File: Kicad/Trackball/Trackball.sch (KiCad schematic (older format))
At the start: 23 parts, among them J1 52559-1233, J10 Conn_01x04_Female, J11 Conn_01x04_Female, J12 Conn_01x04_Female, J13 Conn_01x04_Female, J14 Conn_01x04_Female, J15 Conn_01x04_Female, J16 Conn_01x04_Female, J17 Conn_01x04_Female, J2 Conn_01x04_Male, J3 Conn_01x04_Male, J4 Conn_01x04_Male, J5 Conn_01x04_Male, J6 Conn_01x04_Male, J7 Conn_01x04_Male, J8 Conn_01x04_Male, J9 Conn_01x04_Male, U1 ProMicro

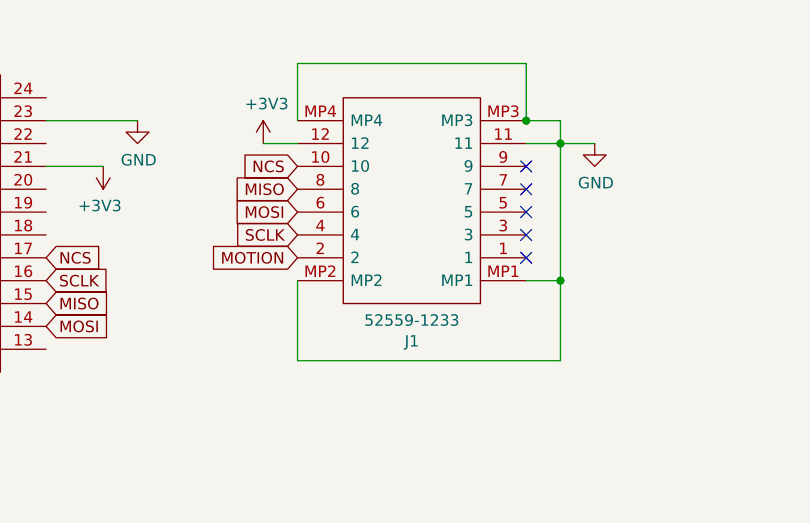
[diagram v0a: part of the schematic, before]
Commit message: Trackball v2: Initial project draft, lot of changes coming.
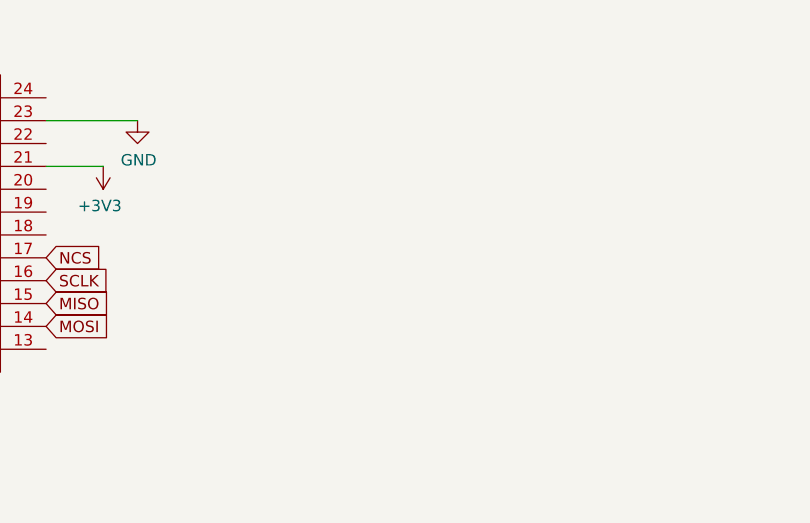
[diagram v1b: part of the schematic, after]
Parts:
- removed J1: 52559-1233, 52559-1233:525591233, symbol 52559-1233:52559-1233
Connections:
- no-connect marks 5 -> 0
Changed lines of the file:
@@
 $EndComp
-$Comp
-L power:+3V3 #PWR0101
-U 1 1 681FE87E
-P 6850 2800
-F 0 "#PWR0101" H 6850 2650 50  0001 C CNN
-F 1 "+3V3" H 6865 2973 50  0000 C CNN
-F 2 "" H 6850 2800 50  0001 C CNN
-F 3 "" H 6850 2800 50  0001 C CNN
-	1    6850 2800
-	1    0    0    -1
-$EndComp
-Wire Wire Line
-	7000 2800 6850 2800
-$Comp
-L power:GND #PWR0102
-U 1 1 68201B1F
-P 8300 2800
-F 0 "#PWR0102" H 8300 2550 50  0001 C CNN
-F 1 "GND" H 8305 2627 50  0000 C CNN
-F 2 "" H 8300 2800 50  0001 C CNN
-F 3 "" H 8300 2800 50  0001 C CNN
-	1    8300 2800
-	1    0    0    -1
-$EndComp
-Text GLabel 7000 2900 0    50   Input ~ 0
-NCS
-Text GLabel 7000 3000 0    50   Input ~ 0
-MISO
-Text GLabel 7000 3100 0    50   Input ~ 0
-MOSI
-Text GLabel 7000 3200 0    50   Input ~ 0
-SCLK
-Text GLabel 7000 3300 0    50   Input ~ 0
-MOTION
-Wire Wire Line
-	8000 3400 8150 3400
-Wire Wire Line
-	8150 2700 8000 2700
-Wire Wire Line
-	8000 2700 8000 2450
-Wire Wire Line
-	8000 2450 7000 2450
-Wire Wire Line
-	7000 2450 7000 2700
-Wire Wire Line
-	7000 3750 8150 3750
-Wire Wire Line
-	8150 3750 8150 3400
 $Comp
 L MX_Alps_Hybrid:MX-NoLED MX4
@@
 	-1   0    0    -1
 $EndComp
-Wire Wire Line
-	8000 2800 8150 2800
-Connection ~ 8150 3400
-Wire Wire Line
-	8150 2700 8150 2800
-Connection ~ 8150 2800
-Wire Wire Line
-	8150 2800 8300 2800
-Wire Wire Line
-	8150 2800 8150 3400
 Text GLabel 4500 2700 0    50   Input ~ 0
 MOTION
@@
 Wire Wire Line
 	5900 2900 6150 2900
-Connection ~ 8000 2700
-Wire Wire Line
-	7000 3400 7000 3750
-$Comp
-L 52559-1233:52559-1233 J1
-U 1 1 681FC9A0
-P 8000 3400
-F 0 "J1" H 8500 3665 50  0000 C CNN
-F 1 "52559-1233" H 8500 3574 50  0000 C CNN
-F 2 "52559-1233:525591233" H 8850 3500 50  0001 L CNN
-F 3 "" H 8850 3400 50  0001 L CNN
-F 4 "FFC & FPC Connectors 0.5 FPC ZIF 12Ckt Sn-Ag-Bi" H 8850 3300 50  0001 L CNN "Description"
-F 5 "5.55" H 8850 3200 50  0001 L CNN "Height"
-F 6 "538-52559-1233" H 8850 3100 50  0001 L CNN "Mouser Part Number"
-F 7 "https://www.mouser.co.uk/ProductDetail/Molex/52559-1233?qs=Q7nJoqLg%252BZgmtCe8OD7vZw%3D%3D" H 8850 3000 50  0001 L CNN "Mouser Price/Stock"
-F 8 "Molex" H 8850 2900 50  0001 L CNN "Manufacturer_Name"
-F 9 "52559-1233" H 8850 2800 50  0001 L CNN "Manufacturer_Part_Number"
-	1    8000 3400
-	-1   0    0    1
-$EndComp
-NoConn ~ 8000 2900
-NoConn ~ 8000 3000
-NoConn ~ 8000 3100
-NoConn ~ 8000 3200
-NoConn ~ 8000 3300
 Wire Wire Line
 	4500 2900 4500 2800
